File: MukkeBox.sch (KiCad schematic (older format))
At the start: 56 parts, among them J101 ST_Link_V2_10P, J102 Jumper, J103 Jumper, J104 Jumper, J105 Jumper, J106 Jumper, J107 PinHeader, J108 PinHeader, J109 PinHeader, Q101 NTK3043N, U101 TPS7B82-Q1, U102 STM32F030C6Tx_MukkeBox, Y101 FOXSDLF/080-20

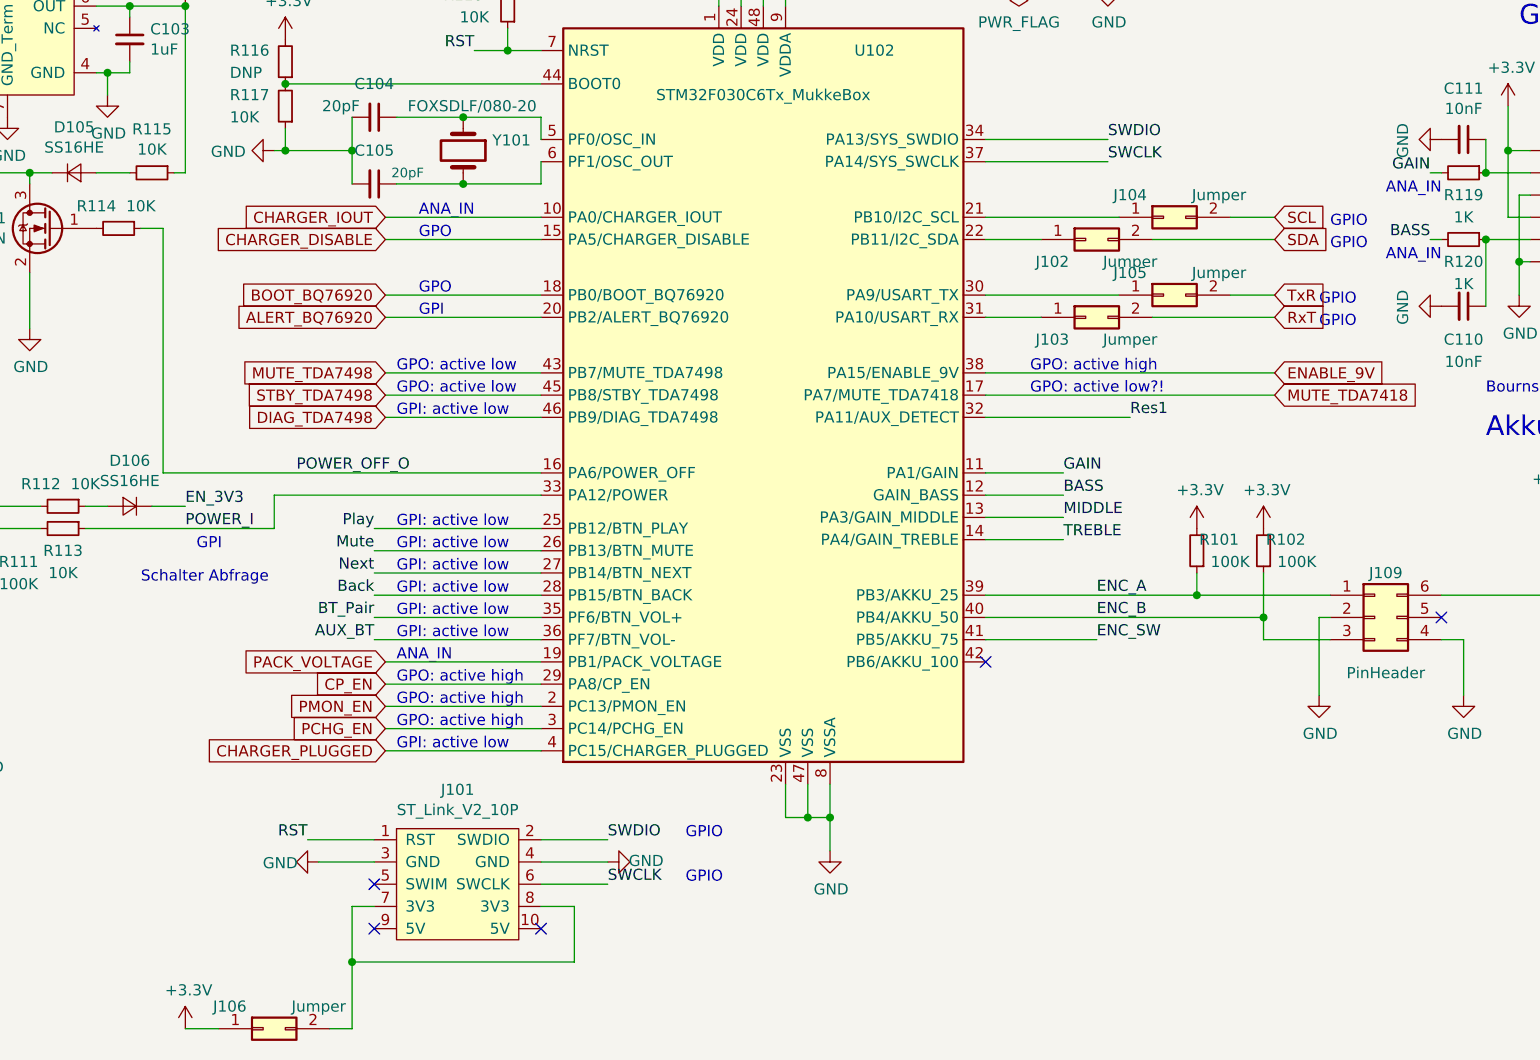
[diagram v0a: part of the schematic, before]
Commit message: fertig zum routen
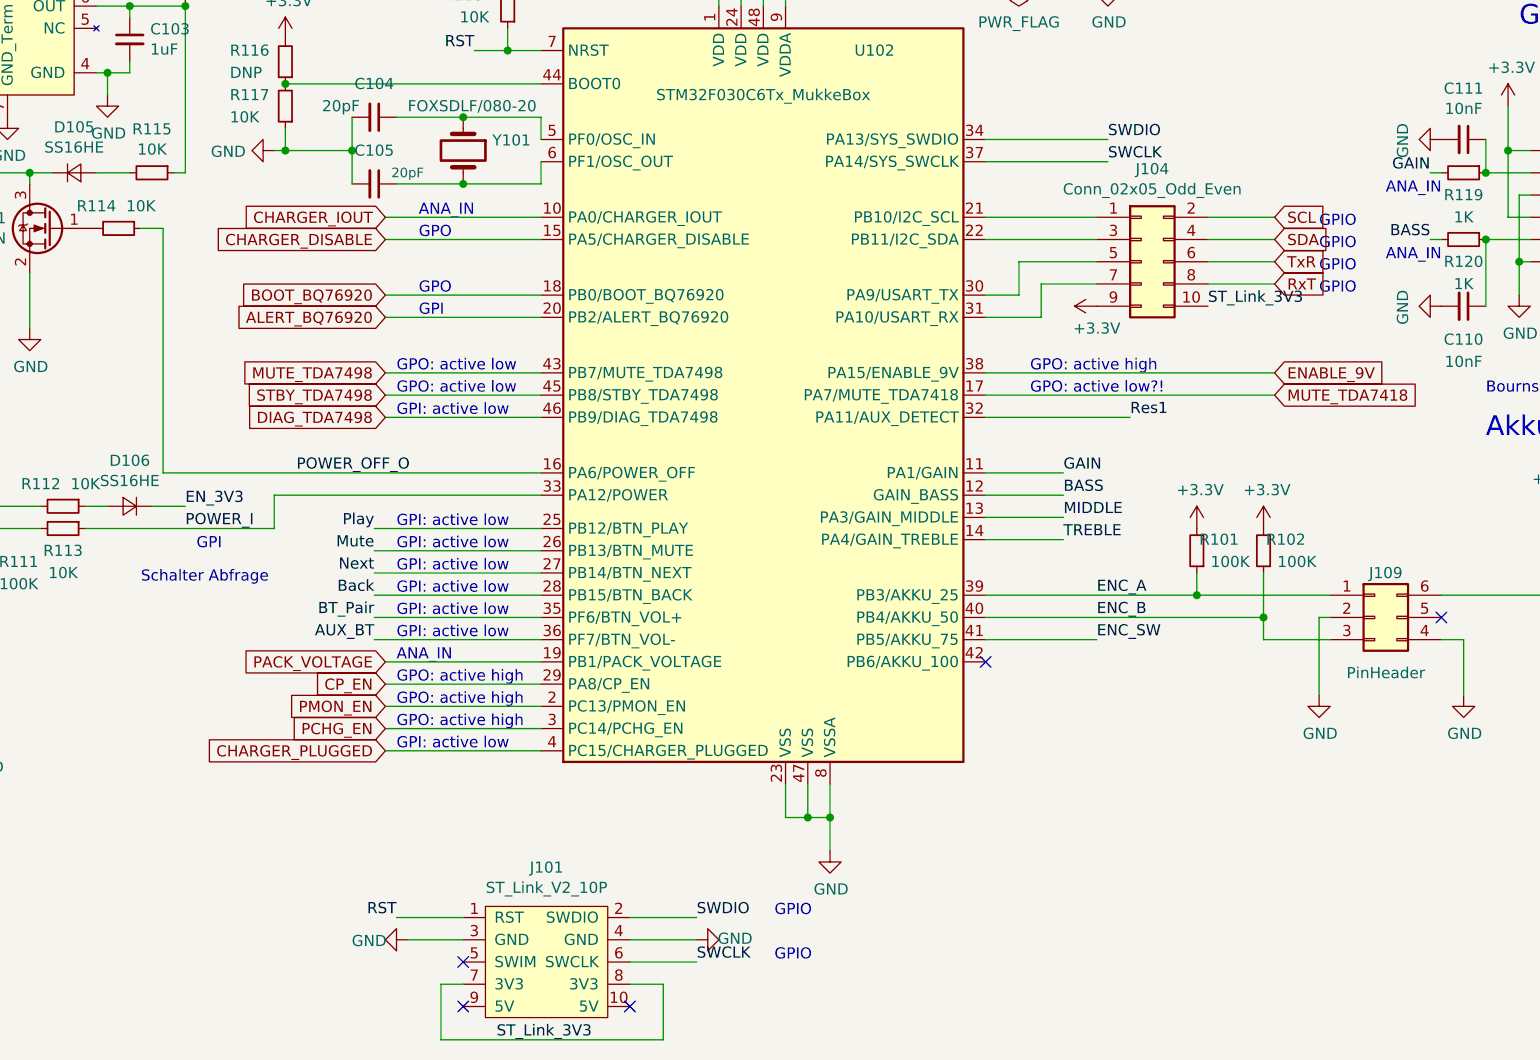
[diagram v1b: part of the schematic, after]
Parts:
- removed J102, J103, J104, J105, J106: Jumper, Connector_PinHeader_2.54mm:PinHeader_1x02_P2.54mm_Vertical, symbol Connector_Generic:Conn_02x01
- added J104: Conn_02x05_Odd_Even, Connector_PinHeader_2.54mm:PinHeader_2x05_P2.54mm_Vertical_SMD, symbol Connector_Generic:Conn_02x05_Odd_Even
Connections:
- net +3V3: now also J104.9 (Pin_9)
- net RxT: now also J104.8 (Pin_8)
- net SCL: now also J104.2 (Pin_2)
- net SDA: now also J104.4 (Pin_4)
- net TxR: now also J104.6 (Pin_6)
- net ST_Link_3V3: now reaches J101.7 (3V3), J101.8 (3V3)
- net ST_Link_3V3: now also J104.10 (Pin_10)
- net at U102.21 (PB10/I2C_SCL): now also J104.1 (Pin_1)
- net at U102.22 (PB11/I2C_SDA): now also J104.3 (Pin_3)
- net at U102.30 (PA9/USART_TX): now also J104.5 (Pin_5)
- net at U102.31 (PA10/USART_RX): now also J104.7 (Pin_7)
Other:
- moved on the sheet: J101
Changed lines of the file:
@@
 L Connector:ST_Link_V2_10P J101
 U 1 1 5E7E5D5D
-P 5100 7000
-F 0 "J101" H 5075 7425 50  0000 C CNN
-F 1 "ST_Link_V2_10P" H 5075 7334 50  0000 C CNN
-F 2 "Connector_PinHeader_2.54mm:PinHeader_2x05_P2.54mm_Vertical" H 5100 7500 50  0001 C CNN
-F 3 "" H 5100 7500 50  0001 C CNN
-	1    5100 7000
+P 5500 7350
+F 0 "J101" H 5475 7775 50  0000 C CNN
+F 1 "ST_Link_V2_10P" H 5475 7684 50  0000 C CNN
+F 2 "Connector_PinHeader_2.54mm:PinHeader_2x05_P2.54mm_Vertical" H 5500 7850 50  0001 C CNN
+F 3 "" H 5500 7850 50  0001 C CNN
+	1    5500 7350
 	1    0    0    -1
 $EndComp
@@
 F1 "Bluetooth.sch" 50
 $EndSheet
-Text GLabel 8750 4450 2    50   Input ~ 0
+Text GLabel 8750 4300 2    50   Input ~ 0
 RxT
-Text GLabel 8750 4350 2    50   Input ~ 0
+Text GLabel 8750 4200 2    50   Input ~ 0
 TxR
 $Comp
@@
 Text Notes 4900 4000 0    50   ~ 0
 ANA_IN
-Text Notes 9000 4050 0    50   ~ 0
+Text Notes 8950 4050 0    50   ~ 0
 GPIO
-Text Notes 9000 4150 0    50   ~ 0
+Text Notes 8950 4150 0    50   ~ 0
 GPIO
-Text Notes 8950 4400 0    50   ~ 0
+Text Notes 8950 4250 0    50   ~ 0
 GPIO
-Text Notes 8950 4500 0    50   ~ 0
+Text Notes 8950 4350 0    50   ~ 0
 GPIO
 Text Notes 3900 5500 0    50   ~ 0
 GPI
-Text Label 5750 6800 0    50   ~ 0
+Text Label 6150 7150 0    50   ~ 0
 SWDIO
-Text Label 5750 7000 0    50   ~ 0
+Text Label 6150 7350 0    50   ~ 0
 SWCLK
 Wire Wire Line
-	5750 7000 5450 7000
-Wire Wire Line
-	5750 6800 5450 6800
-Text Notes 6100 6800 0    50   ~ 0
+	6150 7350 5850 7350
+Wire Wire Line
+	6150 7150 5850 7150
+Text Notes 6500 7150 0    50   ~ 0
 GPIO
-Text Notes 6100 7000 0    50   ~ 0
+Text Notes 6500 7350 0    50   ~ 0
 GPIO
 Text Notes 1550 5650 0    50   ~ 0
@@
 L power:GND #PWR0165
 U 1 1 5EA7CAF7
-P 4450 6900
-F 0 "#PWR0165" H 4450 6650 50  0001 C CNN
-F 1 "GND" V 4455 6727 50  0000 C CNN
-F 2 "" H 4450 6900 50  0001 C CNN
-F 3 "" H 4450 6900 50  0001 C CNN
-	1    4450 6900
-	0    1    1    0
-$EndComp
-Wire Wire Line
-	4700 6900 4450 6900
+P 4850 7250
+F 0 "#PWR0165" H 4850 7000 50  0001 C CNN
+F 1 "GND" V 4855 7077 50  0000 C CNN
+F 2 "" H 4850 7250 50  0001 C CNN
+F 3 "" H 4850 7250 50  0001 C CNN
+	1    4850 7250
+	0    1    1    0
+$EndComp
+Wire Wire Line
+	5100 7250 4850 7250
 $Comp
 L power:GND #PWR0174
 U 1 1 5EA8127F
-P 5750 6900
-F 0 "#PWR0174" H 5750 6650 50  0001 C CNN
-F 1 "GND" V 5755 6727 50  0000 C CNN
-F 2 "" H 5750 6900 50  0001 C CNN
-F 3 "" H 5750 6900 50  0001 C CNN
-	1    5750 6900
+P 6150 7250
+F 0 "#PWR0174" H 6150 7000 50  0001 C CNN
+F 1 "GND" V 6155 7077 50  0000 C CNN
+F 2 "" H 6150 7250 50  0001 C CNN
+F 3 "" H 6150 7250 50  0001 C CNN
+	1    6150 7250
 	0    -1   -1   0
 $EndComp
 Wire Wire Line
-	5750 6900 5450 6900
+	6150 7250 5850 7250
 Text Label 9450 4100 2    50   ~ 0
 BASS
@@
 	1    0    0    -1
 $EndComp
-Text Label 4400 6800 2    50   ~ 0
+Text Label 4800 7150 2    50   ~ 0
 RST
 Wire Wire Line
-	4700 6800 4400 6800
+	5100 7150 4800 7150
 Text Label 5150 3250 2    50   ~ 0
 RST
@@
 Wire Wire Line
 	8750 4800 7450 4800
-$Comp
-L Connector_Generic:Conn_02x01 J103
-U 1 1 5EB922F7
-P 7900 4450
-F 0 "J103" H 7750 4350 50  0000 C CNN
-F 1 "Jumper" H 8100 4350 50  0000 C CNN
-F 2 "Connector_PinHeader_2.54mm:PinHeader_1x02_P2.54mm_Vertical" H 7900 4450 50  0001 C CNN
-F 3 "~" H 7900 4450 50  0001 C CNN
-	1    7900 4450
-	1    0    0    -1
-$EndComp
-$Comp
-L Connector_Generic:Conn_02x01 J105
-U 1 1 5EBA6EA9
-P 8250 4350
-F 0 "J105" H 8100 4450 50  0000 C CNN
-F 1 "Jumper" H 8500 4450 50  0000 C CNN
-F 2 "Connector_PinHeader_2.54mm:PinHeader_1x02_P2.54mm_Vertical" H 8250 4350 50  0001 C CNN
-F 3 "~" H 8250 4350 50  0001 C CNN
-	1    8250 4350
-	1    0    0    -1
-$EndComp
-Wire Wire Line
-	8750 4350 8550 4350
-Wire Wire Line
-	8750 4450 8200 4450
 Wire Wire Line
 	7700 4450 7450 4450
-Wire Wire Line
-	8050 4350 7450 4350
-$Comp
-L Connector_Generic:Conn_02x01 J104
-U 1 1 5EC070B4
-P 8250 4000
-F 0 "J104" H 8100 4100 50  0000 C CNN
-F 1 "Jumper" H 8500 4100 50  0000 C CNN
-F 2 "Connector_PinHeader_2.54mm:PinHeader_1x02_P2.54mm_Vertical" H 8250 4000 50  0001 C CNN
-F 3 "~" H 8250 4000 50  0001 C CNN
-	1    8250 4000
-	1    0    0    -1
-$EndComp
-$Comp
-L Connector_Generic:Conn_02x01 J102
-U 1 1 5EC07148
-P 7900 4100
-F 0 "J102" H 7750 4000 50  0000 C CNN
-F 1 "Jumper" H 8100 4000 50  0000 C CNN
-F 2 "Connector_PinHeader_2.54mm:PinHeader_1x02_P2.54mm_Vertical" H 7900 4100 50  0001 C CNN
-F 3 "~" H 7900 4100 50  0001 C CNN
-	1    7900 4100
-	1    0    0    -1
-$EndComp
-Wire Wire Line
-	8050 4000 7450 4000
-Wire Wire Line
-	7700 4100 7450 4100
-Wire Wire Line
-	8550 4000 8750 4000
-Wire Wire Line
-	8750 4100 8200 4100
 Wire Wire Line
 	4750 4900 5450 4900
@@
 $EndComp
 Connection ~ 6800 2750
-NoConn ~ 5450 7200
-NoConn ~ 4700 7200
-NoConn ~ 4700 7000
-$Comp
-L Connector_Generic:Conn_02x01 J106
-U 1 1 5EB2E486
-P 4200 7650
-F 0 "J106" H 4050 7750 50  0000 C CNN
-F 1 "Jumper" H 4450 7750 50  0000 C CNN
-F 2 "Connector_PinHeader_2.54mm:PinHeader_1x02_P2.54mm_Vertical" H 4200 7650 50  0001 C CNN
-F 3 "~" H 4200 7650 50  0001 C CNN
-	1    4200 7650
-	1    0    0    -1
-$EndComp
-Wire Wire Line
-	5450 7100 5600 7100
-Wire Wire Line
-	5600 7100 5600 7350
-Wire Wire Line
-	5600 7350 4600 7350
-Wire Wire Line
-	4600 7350 4600 7650
-Wire Wire Line
-	4600 7650 4500 7650
-Wire Wire Line
-	4700 7100 4600 7100
-Wire Wire Line
-	4600 7100 4600 7350
-Connection ~ 4600 7350
+NoConn ~ 5850 7550
+NoConn ~ 5100 7550
+NoConn ~ 5100 7350
+Wire Wire Line
+	5850 7450 6000 7450
+Wire Wire Line
+	6000 7450 6000 7700
+Wire Wire Line
+	6000 7700 5000 7700
+Wire Wire Line
+	5100 7450 5000 7450
+Wire Wire Line
+	5000 7450 5000 7700
 $Comp
 L power:+3.3V #PWR0177
 U 1 1 5EB4E6E4
-P 3850 7650
-F 0 "#PWR0177" H 3850 7500 50  0001 C CNN
-F 1 "+3.3V" H 3865 7823 50  0000 C CNN
-F 2 "" H 3850 7650 50  0001 C CNN
-F 3 "" H 3850 7650 50  0001 C CNN
-	1    3850 7650
-	1    0    0    -1
-$EndComp
-Wire Wire Line
-	4000 7650 3850 7650
+P 7950 4400
+F 0 "#PWR0177" H 7950 4250 50  0001 C CNN
+F 1 "+3.3V" V 7850 4400 50  0000 C CNN
+F 2 "" H 7950 4400 50  0001 C CNN
+F 3 "" H 7950 4400 50  0001 C CNN
+	1    7950 4400
+	0    -1   -1   0
+$EndComp
 $Comp
 L power:PWR_FLAG #FLG0101
@@
 Wire Wire Line
 	10150 1000 10150 1200
+Wire Wire Line
+	8750 4100 8450 4100
+Wire Wire Line
+	8450 4200 8750 4200
+Wire Wire Line
+	8450 4300 8750 4300
+Wire Wire Line
+	8450 4000 8750 4000
+Wire Wire Line
+	7950 4000 7450 4000
+Wire Wire Line
+	7450 4100 7950 4100
+Wire Wire Line
+	7950 4200 7600 4200
+Wire Wire Line
+	7600 4200 7600 4350
+Wire Wire Line
+	7600 4350 7450 4350
+Wire Wire Line
+	7950 4300 7700 4300
+Wire Wire Line
+	7700 4300 7700 4450
+Text Label 8450 4400 0    50   ~ 0
+ST_Link_3V3
+Text Label 5250 7700 0    50   ~ 0
+ST_Link_3V3
+$Comp
+L Connector_Generic:Conn_02x05_Odd_Even J104
+U 1 1 5EAA894B
+P 8150 4200
+F 0 "J104" H 8200 4617 50  0000 C CNN
+F 1 "Conn_02x05_Odd_Even" H 8200 4526 50  0000 C CNN
+F 2 "Connector_PinHeader_2.54mm:PinHeader_2x05_P2.54mm_Vertical_SMD" H 8150 4200 50  0001 C CNN
+F 3 "~" H 8150 4200 50  0001 C CNN
+	1    8150 4200
+	1    0    0    -1
+$EndComp
 $EndSCHEMATC
